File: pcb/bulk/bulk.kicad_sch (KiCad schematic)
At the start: 94 parts

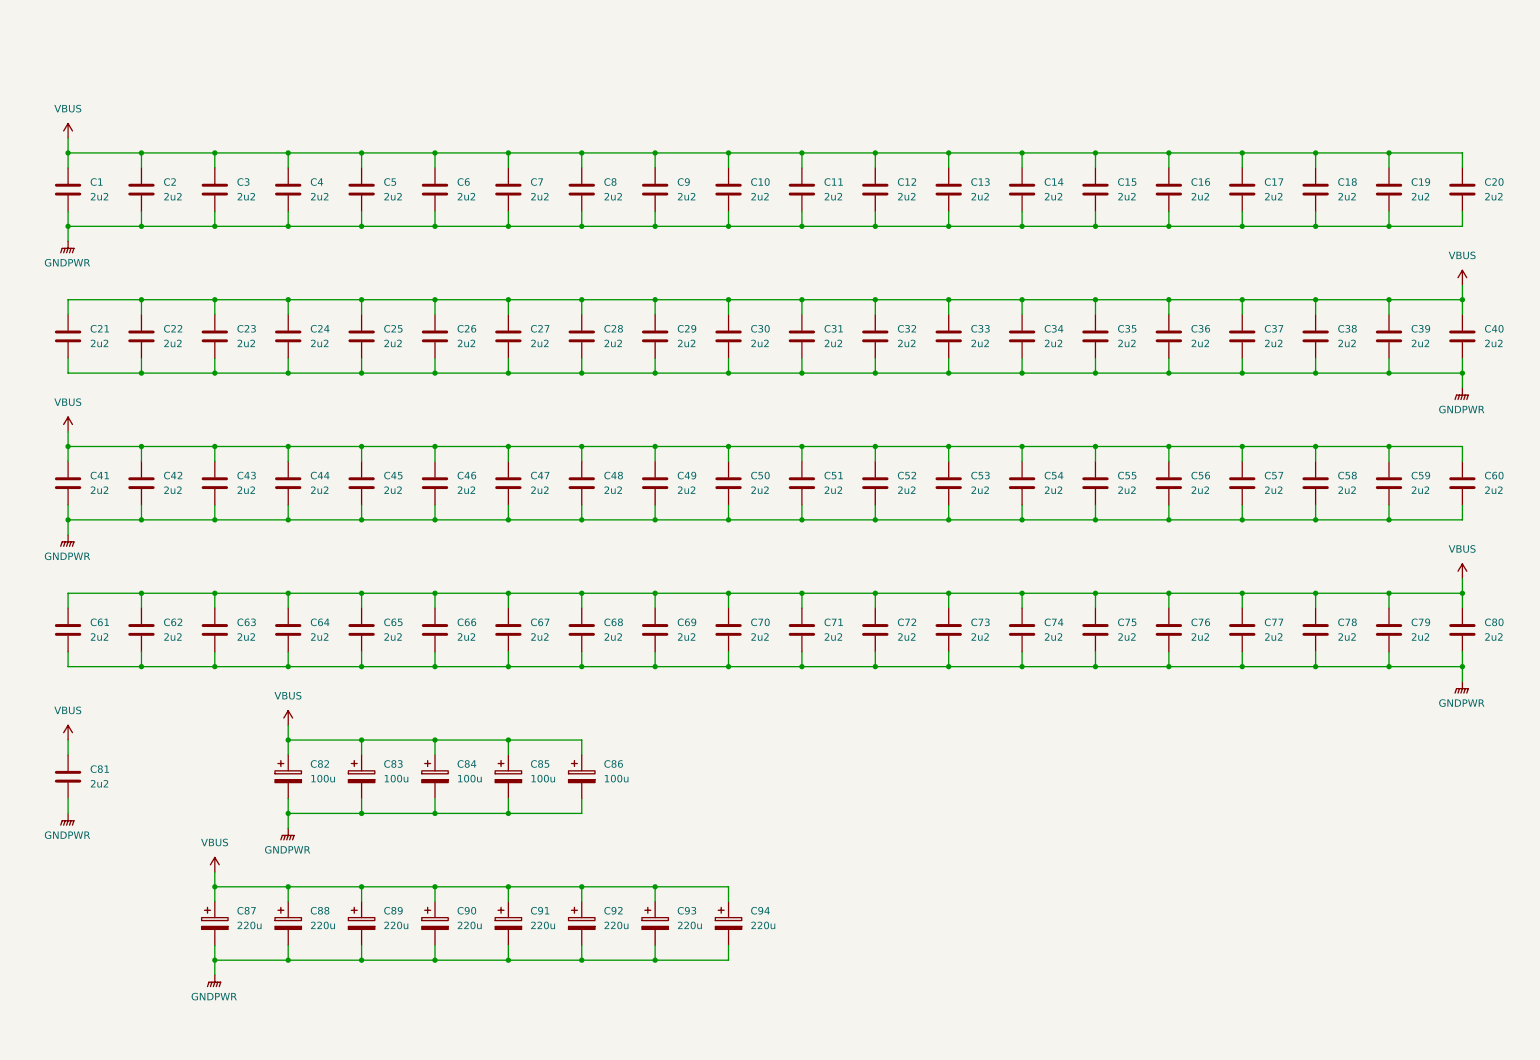
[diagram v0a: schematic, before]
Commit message: Finish rev 1
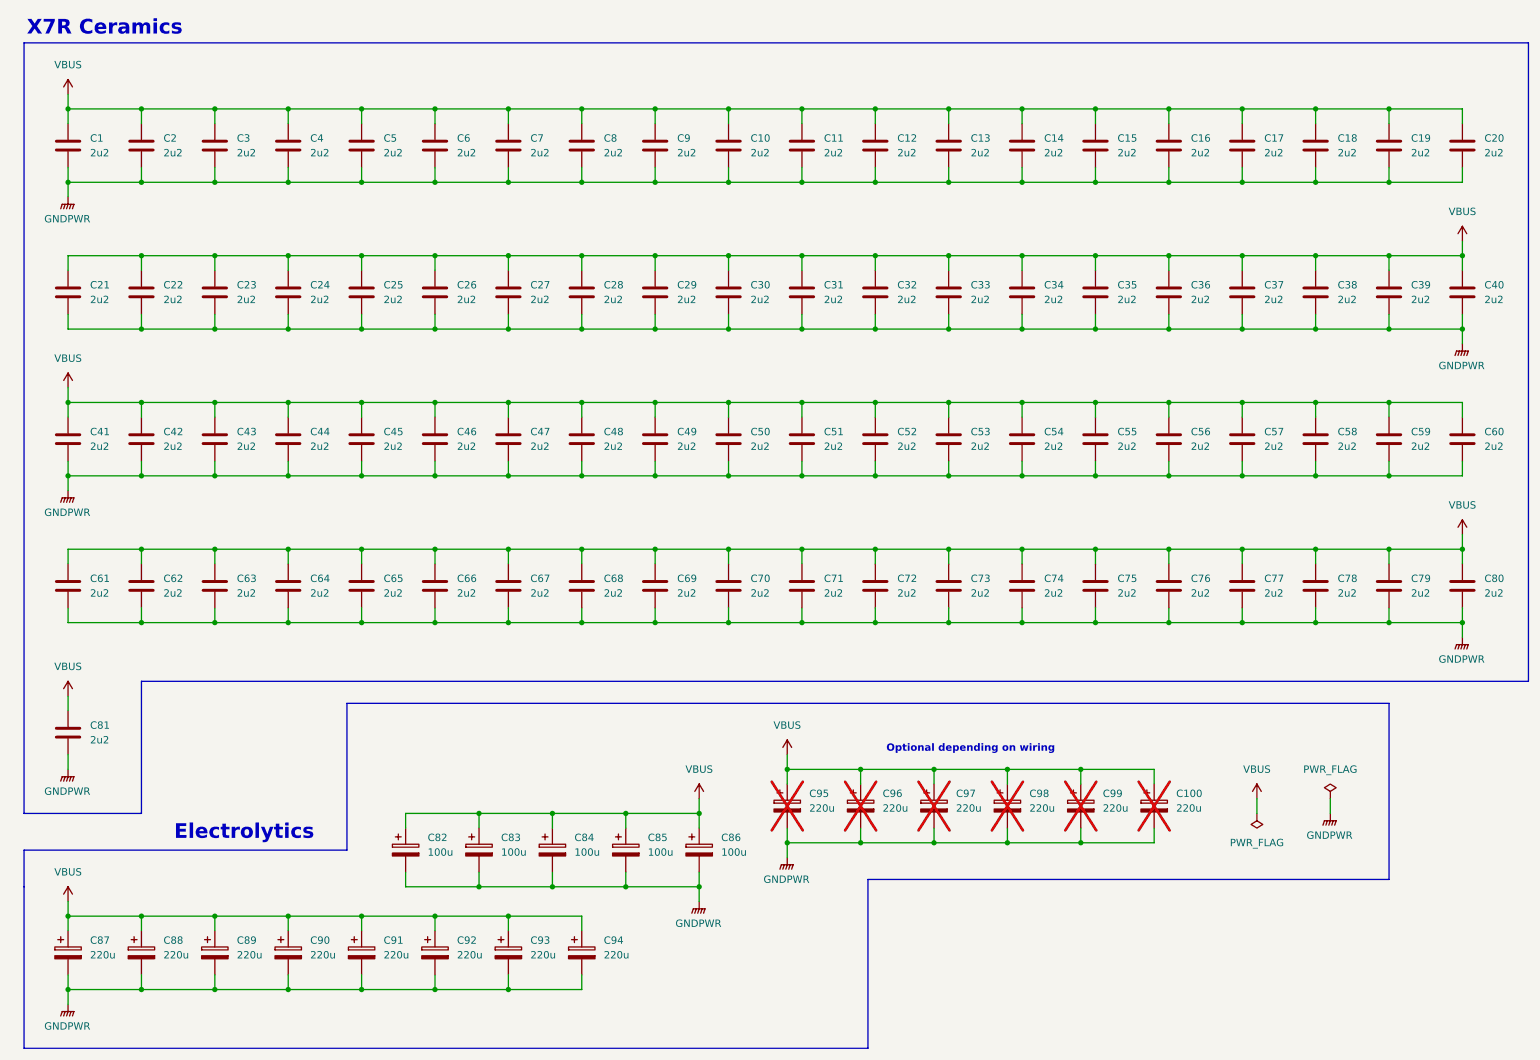
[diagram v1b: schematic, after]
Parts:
- added C100, C95, C96, C97, C98, C99: 220u, Capacitor_THT:C_Radial_D12.5mm_H20.0mm_P5.00mm, symbol Device:C_Polarized
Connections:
- net GNDPWR: now also C100.2, C95.2, C96.2, C97.2, C98.2, C99.2
- net VBUS: now also C100.1, C95.1, C96.1, C97.1, C98.1, C99.1
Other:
- note added: "Electrolytics"
- note added: "Optional depending on wiring"
- note added: "X7R Ceramics"
- moved on the sheet: C1, C10, C11, C12, C13, C14, C15, C16, C17, C18, C19, C2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
